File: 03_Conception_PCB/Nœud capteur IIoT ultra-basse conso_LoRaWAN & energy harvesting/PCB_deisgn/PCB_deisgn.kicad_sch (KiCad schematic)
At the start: 7 parts, among them U1 AEM10941-QFN

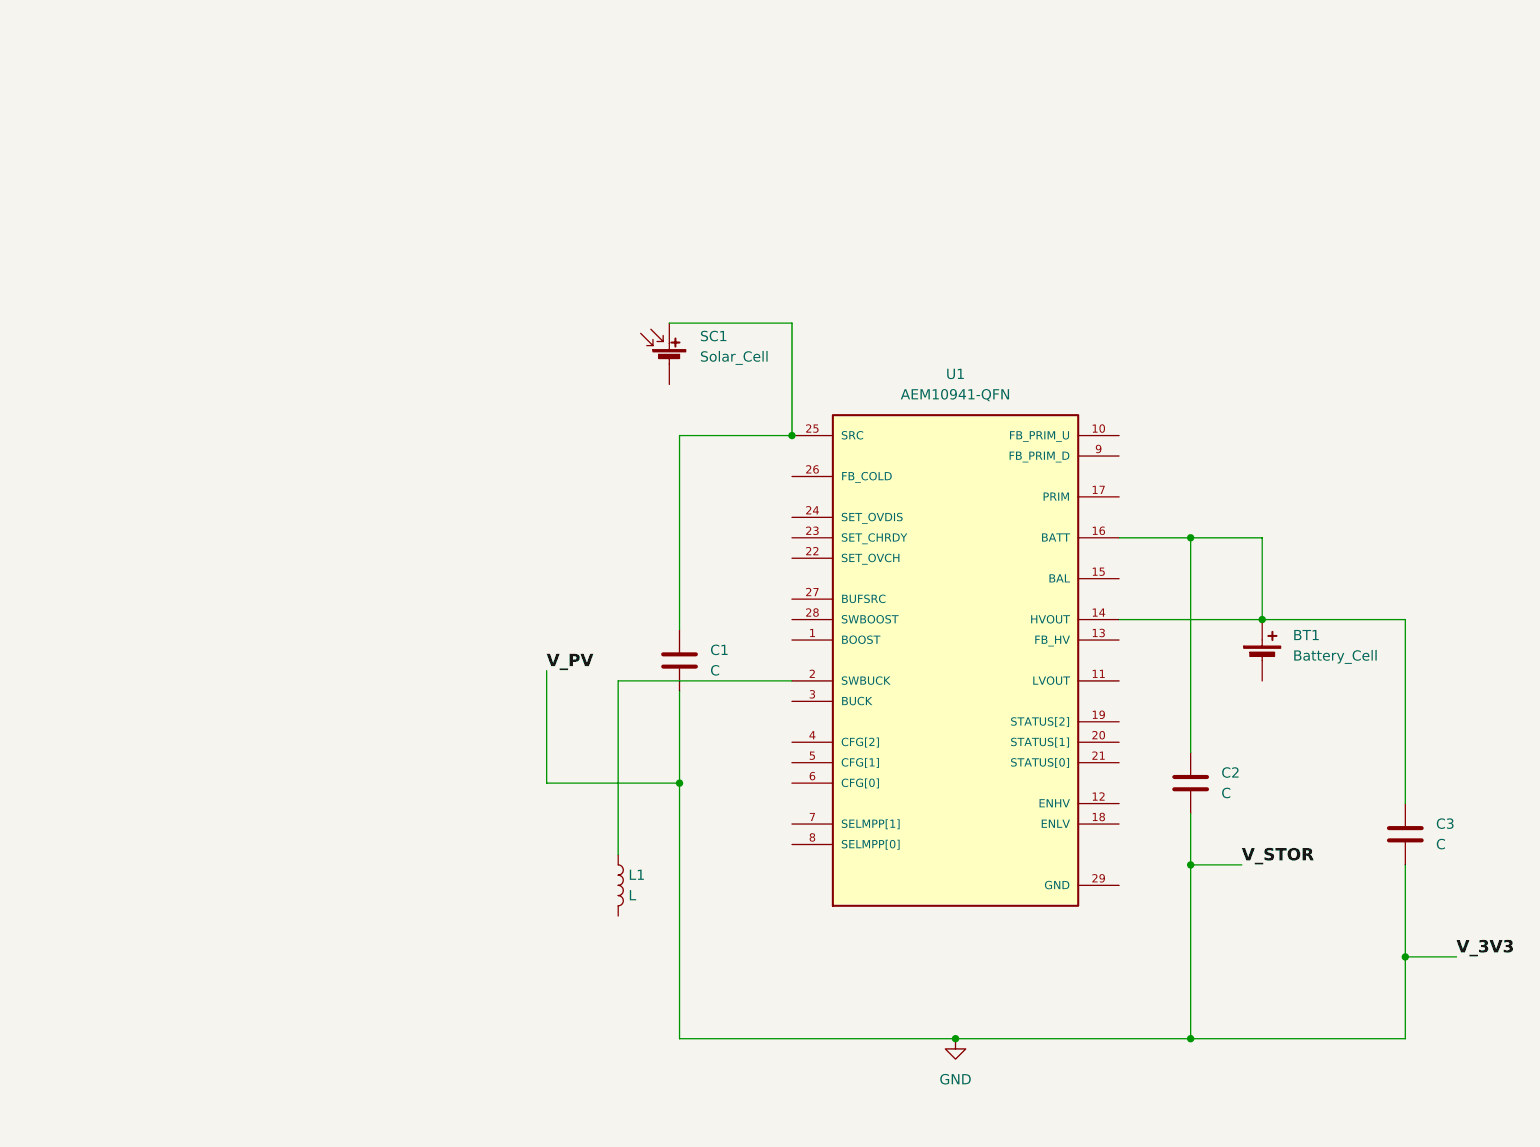
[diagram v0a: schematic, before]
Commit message: Update
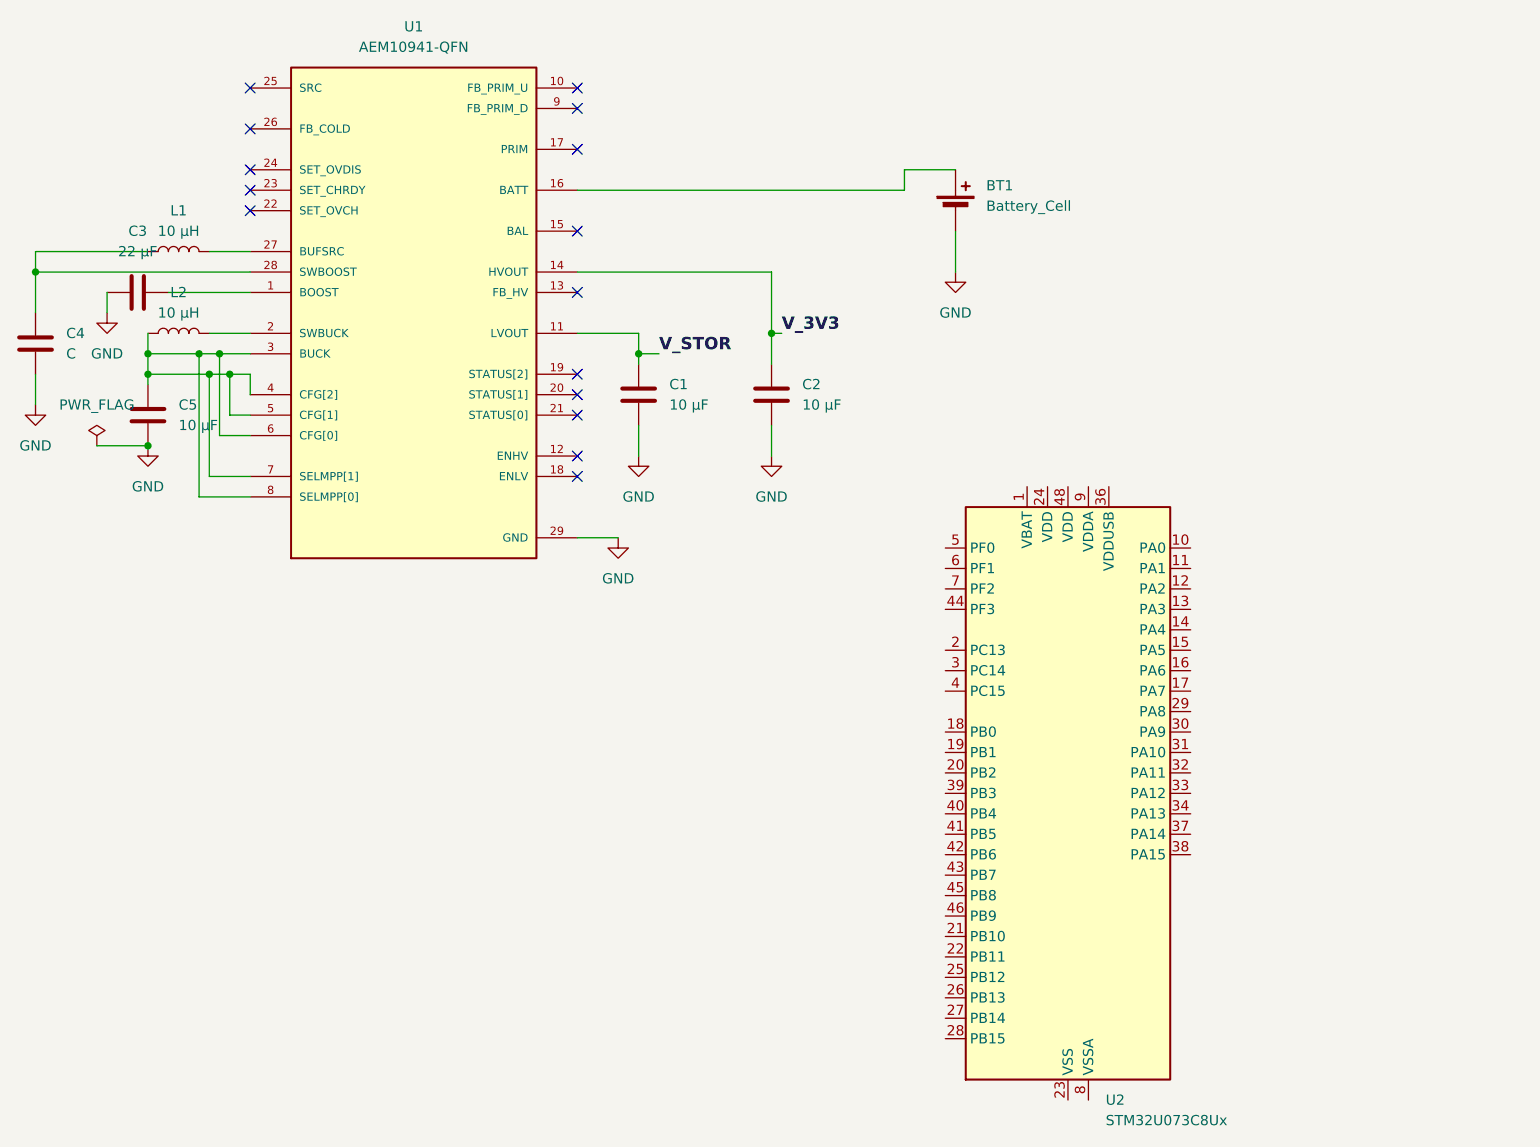
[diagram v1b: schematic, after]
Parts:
- removed SC1: Solar_Cell, symbol Device:Solar_Cell
- added C4: C, symbol Device:C
- added C5: 10 µF, symbol Device:C
- added L2: 10 µH, symbol Device:L
- added U2: STM32U073C8Ux, Package_DFN_QFN:QFN-48-1EP_7x7mm_P0.5mm_EP5.6x5.6mm, symbol MCU_ST_STM32U0:STM32U073C8Ux
- C1, C2: value C -> 10 µF
- C3: value C -> 22 µF
- L1: value L -> 10 µH
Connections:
- net GND: now also BT1.2 (-), U1.29 (GND), C4.1, C5.2
- net at L1.1: now also U1.28 (SWBOOST), C4.2; no longer U1.2 (SWBUCK)
- net at L1.2: now also U1.27 (BUFSRC)
- net at U1.25 (SRC): no longer C1.1
- net at U1.1 (BOOST): now also C3.1
- net V_STOR: now reaches U1.11 (LVOUT)
- net V_STOR: now also C1.1
- net at U1.3 (BUCK): now also U1.4 (CFG[2]), U1.5 (CFG[1]), U1.6 (CFG[0]), U1.7 (SELMPP[1]), U1.8 (SELMPP[0]), C5.1, L2.1
- new net: L2.2, U1.2 (SWBUCK)
- new net: BT1.1 (+), U1.16 (BATT)
- new net: U2.23 (VSS), U2.35 (VSS), U2.47 (VSS), U2.49 (VSS)
- new net V_3V3: C2.1, U1.14 (HVOUT)
- no-connect marks 0 -> 15
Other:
- moved on the sheet: BT1, U1
